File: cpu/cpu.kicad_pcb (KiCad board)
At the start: 2 copper layers, 114.1 x 114.6 mm, 30 parts, among them J1 Conn_01x02, J2 Conn_01x15, J3 Conn_01x08, J4 Conn_01x01_Male, J5 Conn_01x03_Male, J6 Conn_01x02_Male, J7 Conn_01x01_Male, J8 Conn_01x03_Male, J9 Conn_01x02_Male, SW1 SW_Push, U1 W65C02SxP, U2 74HC00, U3 NE555P, U4 74HC14, Y1 Crystal

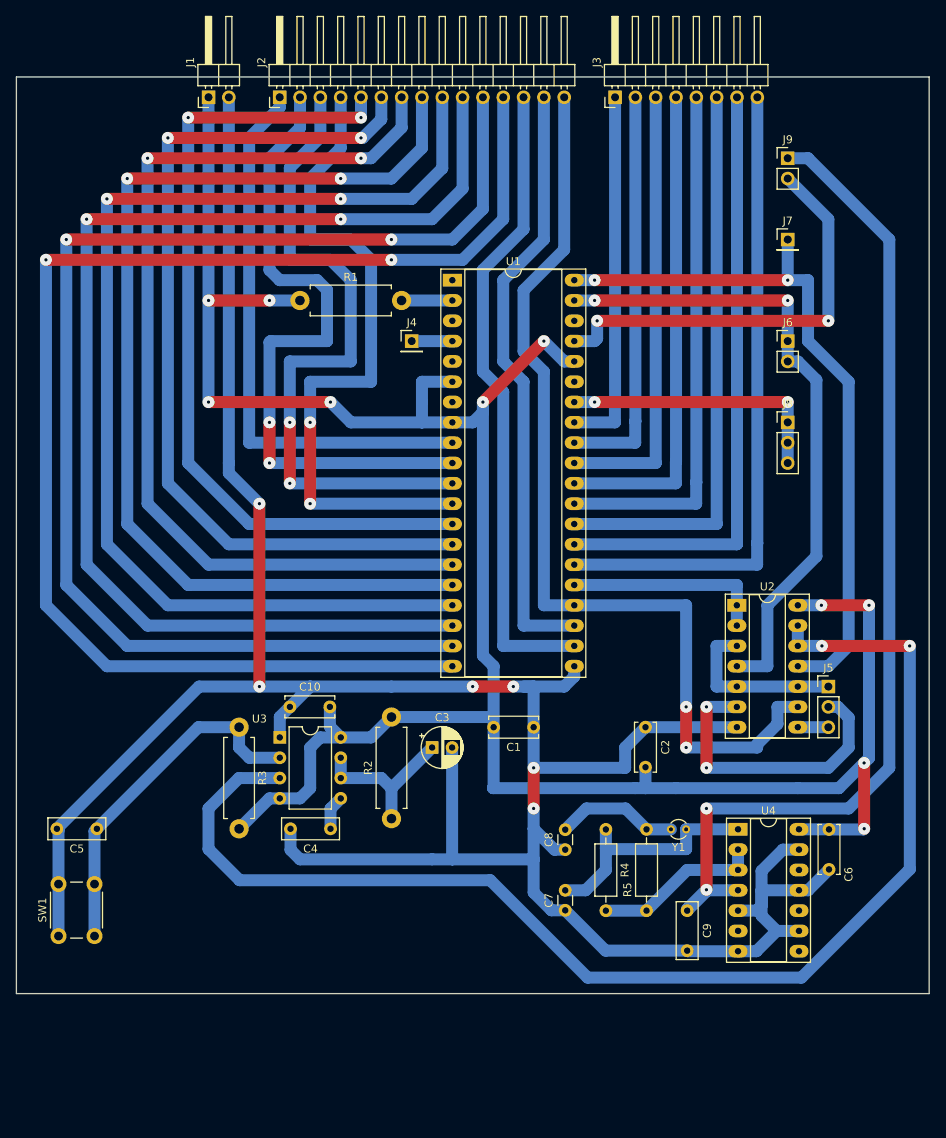
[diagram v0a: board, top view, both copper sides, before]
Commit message: Fit cpu
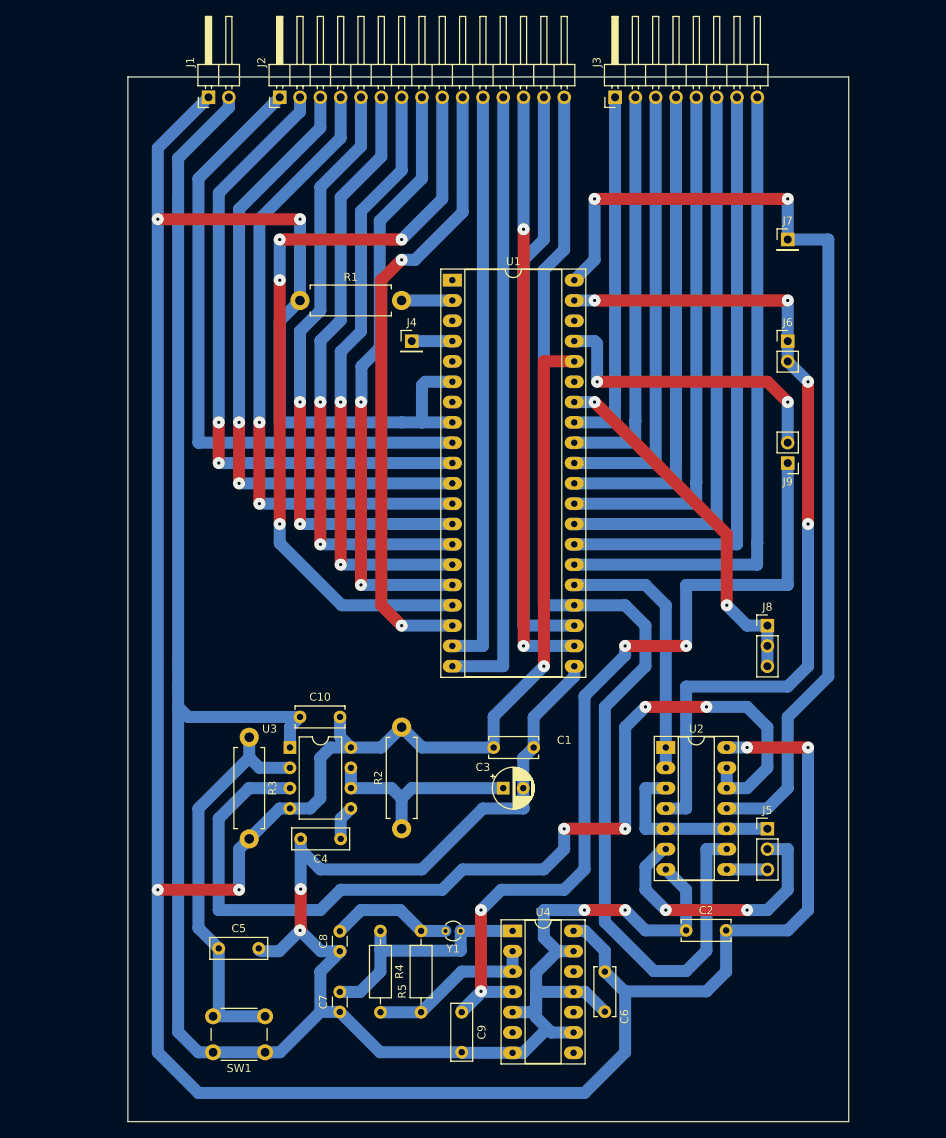
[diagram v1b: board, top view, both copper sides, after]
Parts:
- moved J9 38.1 mm to (111.8, 63.5), turned to 180 degrees
- moved C6 33.2 mm to (88.9, 132.1)
- moved Y1 30.9 mm to (70.9, 122.0)
- moved C7 30.9 mm to (55.8, 132.1)
- moved C8 30.9 mm to (55.8, 124.5)
- moved R4 30.9 mm to (60.9, 122.0)
- moved U4 30.9 mm to (77.4, 122.0)
- moved C9 30.9 mm to (71.0, 132.1)
- moved R5 30.9 mm to (65.9, 132.1)
- moved SW1 29.6 mm to (46.4, 137.2), turned to 180 degrees
- moved C2 25.9 mm to (99.1, 121.9), turned to 0 degrees
- moved J8 25.5 mm to (109.2, 83.8)
- moved C5 21.3 mm to (40.6, 124.2), turned to 0 degrees
- moved U2 19.9 mm to (96.5, 99.1)
- moved J5 19.3 mm to (109.2, 109.2)
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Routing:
- net +5V: track 300.4 -> 454.8 mm, vias 10 -> 7
- net /a11: track 171.6 -> 77.5 mm, vias 2 -> 0
- net /a10: track 162.2 -> 72.4 mm, vias 2 -> 0
- net /a9: track 152.1 -> 78.6 mm
- net /a7: track 131.7 -> 75.5 mm
- net /a6: track 121.6 -> 75.5 mm
- net /a8: track 141.9 -> 97.9 mm, vias 2 -> 4
- net /a5: track 112.3 -> 75.5 mm
- net RESET_PIN: track 89.5 -> 124.9 mm
- net /CLOCK_INV: track 159.9 -> 124.8 mm, vias 2 -> 4
- net A14: track 119.8 -> 149.0 mm, vias 2 -> 0
- net /a4: track 103.5 -> 75.5 mm
- net CLOCK_OUT_PIN: track 81.0 -> 107.5 mm, vias 2 -> 4
- net CLOCK_IN_PIN: track 129.1 -> 109.4 mm, vias 2 -> 4
- net Net-(U1-Pad37): track 54.0 -> 37.7 mm
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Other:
- board size 114.1 x 114.6 mm -> 90.1 x 130.6 mm
